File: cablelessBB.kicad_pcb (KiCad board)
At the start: 2 copper layers, 100 x 60 mm, 306 parts

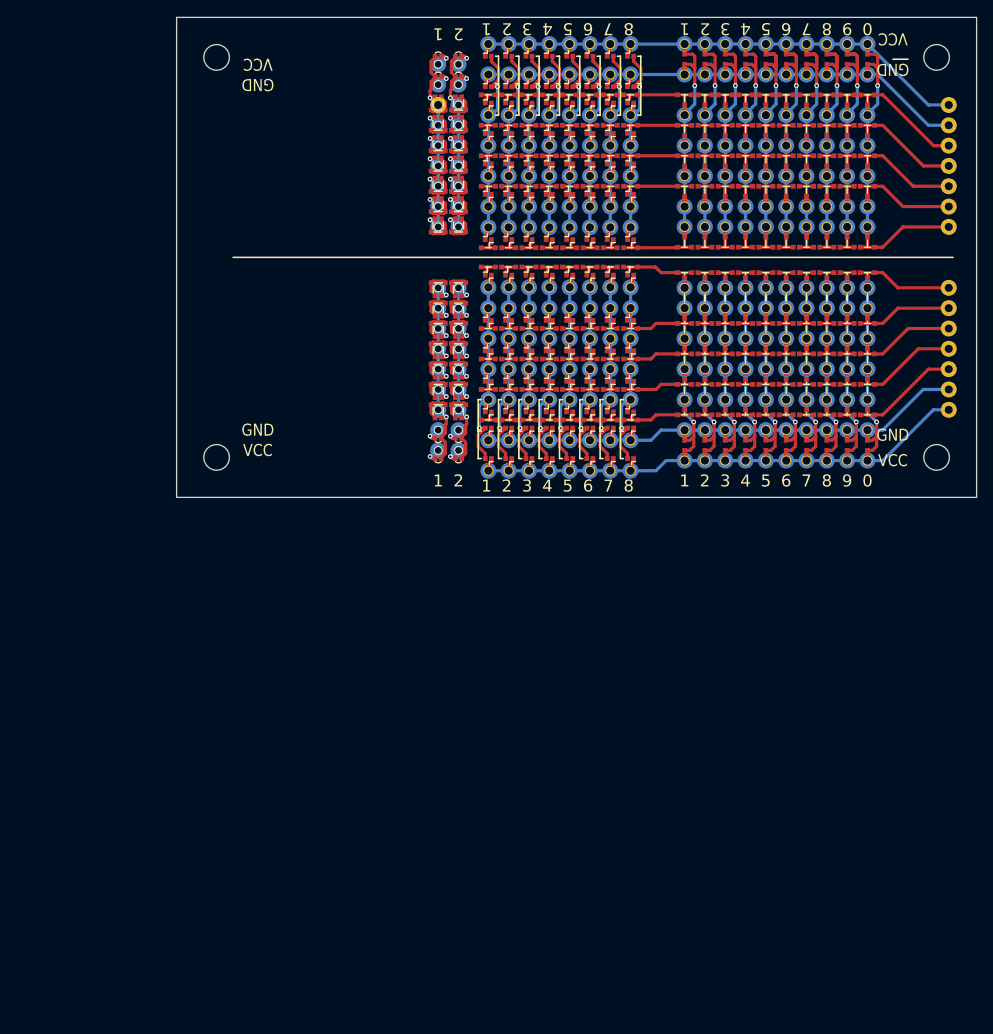
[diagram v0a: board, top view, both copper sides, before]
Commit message: 配線1
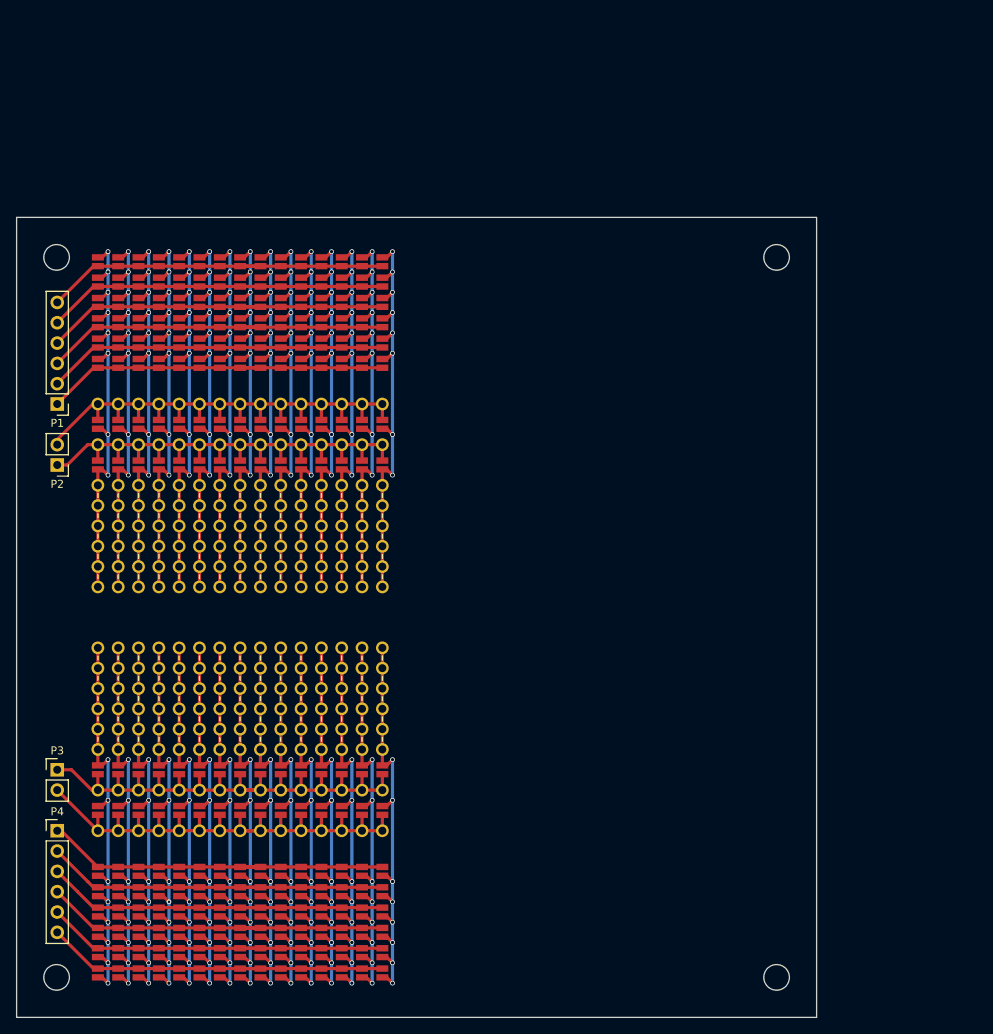
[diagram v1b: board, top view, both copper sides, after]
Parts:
- removed the REF** at (159.0, 72.8)
- removed the REF** at (161.5, 65.2)
- removed the REF** at (174.2, 32.1)
- removed the REF** at (174.2, 41.0)
- removed the REF** at (174.2, 48.6)
- removed the REF** at (174.2, 44.8)
- removed the REF** at (174.2, 51.3)
- removed the REF** at (174.2, 28.3)
- removed the REF** at (176.8, 28.3)
- removed the REF** at (176.8, 51.3)
- removed the REF** at (176.8, 44.8)
- removed the REF** at (176.8, 48.6)
- removed the REF** at (161.5, 61.4)
- removed the REF** at (176.8, 41.0)
- removed the REF** at (216.5, 58.8)
- removed the REF** at (216.5, 61.4)
- removed the REF** at (216.5, 66.4)
- removed the REF** at (216.5, 63.9)
- removed the REF** at (216.5, 74.0)
- removed the REF** at (216.5, 71.5)
- removed the REF** at (216.5, 69.0)
- removed the REF** at (216.5, 46.1)
- removed the REF** at (216.5, 48.6)
- removed the REF** at (161.5, 69.0)
- removed the REF** at (216.5, 51.2)
- removed the REF** at (216.5, 41.0)
- removed the REF** at (216.5, 43.6)
- removed the REF** at (216.5, 38.5)
- removed the REF** at (188.6, 51.2)
- removed the REF** at (188.6, 48.6)
- removed the REF** at (188.6, 44.8)
- removed the REF** at (188.6, 37.2)
- removed the REF** at (188.6, 41.0)
- removed the REF** at (188.6, 32.1)
- removed the REF** at (161.5, 77.9)
- removed the REF** at (201.3, 28.3)
- removed the REF** at (191.1, 41.0)
- removed the REF** at (191.1, 44.8)
- removed the REF** at (191.1, 48.6)
- removed the REF** at (191.1, 51.2)
- removed the REF** at (203.8, 28.3)
- removed the REF** at (191.1, 32.1)
- removed the REF** at (191.1, 37.2)
- removed the REF** at (196.2, 37.2)
- removed the REF** at (196.2, 32.1)
- removed the REF** at (161.5, 72.8)
- removed the REF** at (196.2, 51.2)
- removed the REF** at (196.2, 48.6)
- removed the REF** at (196.2, 44.8)
- removed the REF** at (196.2, 41.0)
- removed the REF** at (193.7, 32.1)
- removed the REF** at (193.7, 41.0)
- removed the REF** at (193.7, 37.2)
- removed the REF** at (193.7, 44.8)
- removed the REF** at (193.7, 48.6)
- removed the REF** at (193.7, 51.2)
- removed the REF** at (166.6, 72.8)
- removed the REF** at (203.8, 51.2)
- removed the REF** at (203.8, 48.6)
- removed the REF** at (203.8, 44.8)
- removed the REF** at (203.8, 37.2)
- removed the REF** at (203.8, 41.0)
- removed the REF** at (203.8, 32.1)
- removed the REF** at (206.4, 41.0)
- removed the REF** at (206.4, 44.8)
- removed the REF** at (206.4, 48.6)
- removed the REF** at (206.4, 51.2)
- removed the REF** at (166.6, 77.9)
- removed the REF** at (206.4, 28.3)
- removed the REF** at (206.4, 32.1)
- removed the REF** at (206.4, 37.2)
- removed the REF** at (201.3, 37.2)
- removed the REF** at (201.3, 32.1)
- removed the REF** at (201.3, 51.2)
- removed the REF** at (201.3, 48.6)
- removed the REF** at (201.3, 44.8)
- removed the REF** at (201.3, 41.0)
- removed the REF** at (198.7, 32.1)
- removed the REF** at (166.6, 69.0)
- removed the REF** at (198.7, 41.0)
- removed the REF** at (198.7, 37.2)
- removed the REF** at (198.7, 44.8)
- removed the REF** at (198.7, 48.6)
- removed the REF** at (198.7, 51.2)
- removed the REF** at (191.1, 28.3)
- removed the REF** at (193.7, 28.3)
- removed the REF** at (186.0, 37.2)
- removed the REF** at (186.0, 32.1)
- removed the REF** at (198.7, 28.3)
- removed the REF** at (166.6, 61.4)
- removed the REF** at (186.0, 51.2)
- removed the REF** at (186.0, 48.6)
- removed the REF** at (186.0, 44.8)
- removed the REF** at (186.0, 41.0)
- removed the REF** at (196.2, 28.3)
- removed the REF** at (183.5, 32.1)
- removed the REF** at (183.5, 41.0)
- removed the REF** at (183.5, 37.2)
- removed the REF** at (183.5, 44.8)
- removed the REF** at (183.5, 48.6)
- removed the REF** at (166.6, 65.2)
- removed the REF** at (183.5, 51.2)
- removed the REF** at (186.0, 28.3)
- removed the REF** at (188.6, 28.3)
- removed the REF** at (183.5, 28.3)
- removed the REF** at (188.6, 76.6)
- removed the REF** at (188.6, 80.4)
- removed the REF** at (191.1, 80.4)
- removed the REF** at (191.1, 76.6)
- removed the REF** at (196.2, 76.6)
- removed the REF** at (196.2, 80.4)
- removed the REF** at (159.0, 77.9)
- removed the REF** at (166.6, 58.7)
- removed the REF** at (193.7, 80.4)
- removed the REF** at (193.7, 76.6)
- removed the REF** at (203.8, 76.6)
- removed the REF** at (203.8, 80.4)
- removed the REF** at (206.4, 80.4)
- removed the REF** at (206.4, 76.6)
- removed the REF** at (201.3, 76.6)
- removed the REF** at (201.3, 80.4)
- removed the REF** at (198.7, 80.4)
- removed the REF** at (198.7, 76.6)
- removed the REF** at (166.6, 81.7)
- removed the REF** at (186.0, 76.6)
- removed the REF** at (186.0, 80.4)
- removed the REF** at (183.5, 80.4)
- removed the REF** at (183.5, 76.6)
- removed the REF** at (188.6, 58.8)
- removed the REF** at (188.6, 61.4)
- removed the REF** at (164.1, 81.7)
- removed the REF** at (188.6, 65.2)
- removed the REF** at (188.6, 72.8)
- removed the REF** at (188.6, 69.0)
- removed the REF** at (191.1, 69.0)
- removed the REF** at (191.1, 72.8)
- removed the REF** at (191.1, 65.2)
- removed the REF** at (191.1, 61.4)
- removed the REF** at (191.1, 58.8)
- removed the REF** at (196.2, 58.8)
- removed the REF** at (196.2, 61.4)
- removed the REF** at (164.1, 58.7)
- removed the REF** at (196.2, 65.2)
- removed the REF** at (196.2, 72.8)
- removed the REF** at (196.2, 69.0)
- removed the REF** at (193.7, 69.0)
- removed the REF** at (193.7, 72.8)
- removed the REF** at (193.7, 65.2)
- removed the REF** at (193.7, 61.4)
- removed the REF** at (193.7, 58.8)
- removed the REF** at (203.8, 58.8)
- removed the REF** at (203.8, 61.4)
- removed the REF** at (164.1, 65.2)
- removed the REF** at (203.8, 65.2)
- removed the REF** at (203.8, 72.8)
- removed the REF** at (203.8, 69.0)
- removed the REF** at (206.4, 69.0)
- removed the REF** at (206.4, 72.8)
- removed the REF** at (206.4, 65.2)
- removed the REF** at (206.4, 61.4)
- removed the REF** at (206.4, 58.8)
- removed the REF** at (201.3, 58.8)
- removed the REF** at (201.3, 61.4)
- removed the REF** at (164.1, 61.4)
- removed the REF** at (201.3, 65.2)
- removed the REF** at (201.3, 72.8)
- removed the REF** at (201.3, 69.0)
- removed the REF** at (198.7, 69.0)
- removed the REF** at (198.7, 72.8)
- removed the REF** at (198.7, 65.2)
- removed the REF** at (198.7, 61.4)
- removed the REF** at (198.7, 58.8)
- removed the REF** at (186.0, 58.8)
- removed the REF** at (186.0, 61.4)
- removed the REF** at (164.1, 69.0)
- removed the REF** at (186.0, 65.2)
- removed the REF** at (186.0, 72.8)
- removed the REF** at (186.0, 69.0)
- removed the REF** at (183.5, 69.0)
- removed the REF** at (183.5, 72.8)
- removed the REF** at (183.5, 65.2)
- removed the REF** at (183.5, 61.4)
- removed the REF** at (183.5, 58.8)
- removed the REF** at (216.5, 36.0)
- removed the REF** at (152.7, 46.1)
- removed the REF** at (164.1, 77.9)
- removed the REF** at (152.7, 48.6)
- removed the REF** at (152.7, 38.5)
- removed the REF** at (152.7, 36.0)
- removed the REF** at (152.7, 41.0)
- removed the REF** at (152.7, 43.6)
- removed the REF** at (152.7, 51.2)
- removed the REF** at (155.2, 51.2)
- removed the REF** at (155.2, 43.6)
- removed the REF** at (155.2, 41.0)
- removed the REF** at (155.2, 36.0)
- removed the REF** at (164.1, 72.8)
- removed the REF** at (155.2, 38.5)
- removed the REF** at (155.2, 48.6)
- removed the REF** at (155.2, 46.1)
- removed the REF** at (155.2, 63.9)
- removed the REF** at (155.2, 61.4)
- removed the REF** at (155.2, 71.5)
- removed the REF** at (155.2, 74.0)
- removed the REF** at (155.2, 69.0)
- removed the REF** at (155.2, 66.4)
- removed the REF** at (155.2, 58.8)
- removed the REF** at (174.2, 72.8)
- removed the REF** at (152.7, 58.8)
- removed the REF** at (152.7, 66.4)
- removed the REF** at (152.7, 69.0)
- removed the REF** at (152.7, 74.0)
- removed the REF** at (152.7, 71.5)
- removed the REF** at (152.7, 61.4)
- removed the REF** at (152.7, 63.9)
- removed the REF** at (152.7, 33.4)
- removed the REF** at (152.7, 30.9)
- removed the REF** at (155.2, 30.9)
- removed the REF** at (159.0, 69.0)
- removed the REF** at (174.2, 77.9)
- removed the REF** at (155.2, 33.4)
- removed the REF** at (155.2, 76.6)
- removed the REF** at (155.2, 79.1)
- removed the REF** at (152.7, 79.1)
- removed the REF** at (152.7, 76.6)
- removed the REF** at (176.8, 32.1)
- removed the REF** at (176.8, 37.2)
- removed the REF** at (174.2, 69.0)
- removed the REF** at (174.2, 61.4)
- removed the REF** at (174.2, 65.2)
- removed the REF** at (174.2, 58.7)
- removed the REF** at (174.2, 81.7)
- removed the REF** at (176.8, 81.7)
- removed the REF** at (176.8, 58.7)
- removed the REF** at (176.8, 65.2)
- removed the REF** at (176.8, 61.4)
- removed the REF** at (159.0, 61.4)
- removed the REF** at (176.8, 69.0)
- removed the REF** at (176.8, 77.9)
- removed the REF** at (176.8, 72.8)
- removed the REF** at (171.7, 72.8)
- removed the REF** at (171.7, 77.9)
- removed the REF** at (171.7, 69.0)
- removed the REF** at (171.7, 61.4)
- removed the REF** at (171.7, 65.2)
- removed the REF** at (171.7, 58.7)
- removed the REF** at (171.7, 81.7)
- removed the REF** at (159.0, 65.2)
- removed the REF** at (169.1, 81.7)
- removed the REF** at (169.1, 58.7)
- removed the REF** at (169.1, 65.2)
- removed the REF** at (169.1, 61.4)
- removed the REF** at (169.1, 69.0)
- removed the REF** at (169.1, 77.9)
- removed the REF** at (169.1, 72.8)
- removed the REF** at (166.6, 37.2)
- removed the REF** at (166.6, 32.1)
- removed the REF** at (166.6, 41.0)
- removed the REF** at (159.0, 58.7)
- removed the REF** at (166.6, 48.6)
- removed the REF** at (166.6, 44.8)
- removed the REF** at (166.6, 51.3)
- removed the REF** at (166.6, 28.3)
- removed the REF** at (164.1, 28.3)
- removed the REF** at (164.1, 51.3)
- removed the REF** at (164.1, 44.8)
- removed the REF** at (164.1, 48.6)
- removed the REF** at (164.1, 41.0)
- removed the REF** at (164.1, 32.1)
- removed the REF** at (159.0, 81.7)
- removed the REF** at (164.1, 37.2)
- removed the REF** at (159.0, 37.2)
- removed the REF** at (159.0, 32.1)
- removed the REF** at (159.0, 41.0)
- removed the REF** at (159.0, 48.6)
- removed the REF** at (159.0, 44.8)
- removed the REF** at (159.0, 51.3)
- removed the REF** at (159.0, 28.3)
- removed the REF** at (161.5, 28.3)
- removed the REF** at (161.5, 51.3)
- removed the REF** at (161.5, 81.7)
- removed the REF** at (161.5, 44.8)
- removed the REF** at (161.5, 48.6)
- removed the REF** at (161.5, 41.0)
- removed the REF** at (161.5, 32.1)
- removed the REF** at (161.5, 37.2)
- removed the REF** at (171.7, 37.2)
- removed the REF** at (171.7, 32.1)
- removed the REF** at (171.7, 41.0)
- removed the REF** at (171.7, 48.6)
- removed the REF** at (171.7, 44.8)
- removed the REF** at (161.5, 58.7)
- removed the REF** at (171.7, 51.3)
- removed the REF** at (171.7, 28.3)
- removed the REF** at (169.1, 28.3)
- removed the REF** at (169.1, 51.3)
- removed the REF** at (169.1, 44.8)
- removed the REF** at (169.1, 48.6)
- removed the REF** at (169.1, 41.0)
- removed the REF** at (169.1, 32.1)
- removed the REF** at (169.1, 37.2)
- removed the REF** at (174.2, 37.2)
- added JP1: Jumper_NO_Small, lib:jump, F.Cu at (110.2, 55.5)
- added JP10: Jumper_NO_Small, lib:jump, F.Cu at (110.2, 124.1)
- added JP100: Jumper_NO_Small, lib:jump, F.Cu at (125.4, 63.2)
- added JP101: Jumper_NO_Small, lib:jump, F.Cu at (125.4, 65.7)
- added JP102: Jumper_NO_Small, lib:jump, F.Cu at (125.4, 68.2)
- added JP103: Jumper_NO_Small, lib:jump, F.Cu at (125.4, 75.9)
- added JP104: Jumper_NO_Small, lib:jump, F.Cu at (125.4, 81.0)
- added JP105: Jumper_NO_Small, lib:jump, F.Cu at (125.4, 119.0)
- added JP106: Jumper_NO_Small, lib:jump, F.Cu at (125.4, 124.1)
- added JP107: Jumper_NO_Small, lib:jump, F.Cu at (125.4, 131.8)
- added JP108: Jumper_NO_Small, lib:jump, F.Cu at (125.4, 134.3)
- added JP109: Jumper_NO_Small, lib:jump, F.Cu at (125.4, 136.8)
- added JP11: Jumper_NO_Small, lib:jump, F.Cu at (110.2, 131.8)
- added JP110: Jumper_NO_Small, lib:jump, F.Cu at (125.4, 139.4)
- added JP111: Jumper_NO_Small, lib:jump, F.Cu at (125.4, 141.9)
- added JP112: Jumper_NO_Small, lib:jump, F.Cu at (125.4, 144.4)
- added JP113: Jumper_NO_Small, lib:jump, F.Cu at (127.9, 55.5)
- added JP114: Jumper_NO_Small, lib:jump, F.Cu at (127.9, 58.1)
- added JP115: Jumper_NO_Small, lib:jump, F.Cu at (127.9, 60.6)
- added JP116: Jumper_NO_Small, lib:jump, F.Cu at (127.9, 63.2)
- added JP117: Jumper_NO_Small, lib:jump, F.Cu at (127.9, 65.7)
- added JP118: Jumper_NO_Small, lib:jump, F.Cu at (127.9, 68.2)
- added JP119: Jumper_NO_Small, lib:jump, F.Cu at (127.9, 75.9)
- added JP12: Jumper_NO_Small, lib:jump, F.Cu at (110.2, 134.3)
- added JP120: Jumper_NO_Small, lib:jump, F.Cu at (127.9, 81.0)
- added JP121: Jumper_NO_Small, lib:jump, F.Cu at (127.9, 119.0)
- added JP122: Jumper_NO_Small, lib:jump, F.Cu at (127.9, 124.1)
- added JP123: Jumper_NO_Small, lib:jump, F.Cu at (127.9, 131.8)
- added JP124: Jumper_NO_Small, lib:jump, F.Cu at (127.9, 134.3)
- added JP125: Jumper_NO_Small, lib:jump, F.Cu at (127.9, 136.8)
- added JP126: Jumper_NO_Small, lib:jump, F.Cu at (127.9, 139.4)
- added JP127: Jumper_NO_Small, lib:jump, F.Cu at (127.9, 141.9)
- added JP128: Jumper_NO_Small, lib:jump, F.Cu at (127.9, 144.4)
- added JP129: Jumper_NO_Small, lib:jump, F.Cu at (130.5, 55.5)
- added JP13: Jumper_NO_Small, lib:jump, F.Cu at (110.2, 136.8)
- added JP130: Jumper_NO_Small, lib:jump, F.Cu at (130.5, 58.1)
- added JP131: Jumper_NO_Small, lib:jump, F.Cu at (130.5, 60.6)
- added JP132: Jumper_NO_Small, lib:jump, F.Cu at (130.5, 63.2)
- added JP133: Jumper_NO_Small, lib:jump, F.Cu at (130.5, 65.7)
- added JP134: Jumper_NO_Small, lib:jump, F.Cu at (130.5, 68.2)
- added JP135: Jumper_NO_Small, lib:jump, F.Cu at (130.5, 75.9)
- added JP136: Jumper_NO_Small, lib:jump, F.Cu at (130.5, 81.0)
- added JP137: Jumper_NO_Small, lib:jump, F.Cu at (130.5, 119.0)
- added JP138: Jumper_NO_Small, lib:jump, F.Cu at (130.5, 124.1)
- added JP139: Jumper_NO_Small, lib:jump, F.Cu at (130.5, 131.8)
- added JP14: Jumper_NO_Small, lib:jump, F.Cu at (110.2, 139.4)
- added JP140: Jumper_NO_Small, lib:jump, F.Cu at (130.5, 134.3)
- added JP141: Jumper_NO_Small, lib:jump, F.Cu at (130.5, 136.8)
- added JP142: Jumper_NO_Small, lib:jump, F.Cu at (130.5, 139.4)
- added JP143: Jumper_NO_Small, lib:jump, F.Cu at (130.5, 141.9)
- added JP144: Jumper_NO_Small, lib:jump, F.Cu at (130.5, 144.4)
- added JP145: Jumper_NO_Small, lib:jump, F.Cu at (133.0, 55.5)
- added JP146: Jumper_NO_Small, lib:jump, F.Cu at (133.0, 58.1)
- added JP147: Jumper_NO_Small, lib:jump, F.Cu at (133.0, 60.6)
- added JP148: Jumper_NO_Small, lib:jump, F.Cu at (133.0, 63.2)
- added JP149: Jumper_NO_Small, lib:jump, F.Cu at (133.0, 65.7)
- added JP15: Jumper_NO_Small, lib:jump, F.Cu at (110.2, 141.9)
- added JP150: Jumper_NO_Small, lib:jump, F.Cu at (133.0, 68.2)
- added JP151: Jumper_NO_Small, lib:jump, F.Cu at (133.0, 75.9)
- added JP152: Jumper_NO_Small, lib:jump, F.Cu at (133.0, 81.0)
- added JP153: Jumper_NO_Small, lib:jump, F.Cu at (133.0, 119.0)
- added JP154: Jumper_NO_Small, lib:jump, F.Cu at (133.0, 124.1)
- added JP155: Jumper_NO_Small, lib:jump, F.Cu at (133.0, 131.8)
- added JP156: Jumper_NO_Small, lib:jump, F.Cu at (133.0, 134.3)
- added JP157: Jumper_NO_Small, lib:jump, F.Cu at (133.0, 136.8)
- added JP158: Jumper_NO_Small, lib:jump, F.Cu at (133.0, 139.4)
- added JP159: Jumper_NO_Small, lib:jump, F.Cu at (133.0, 141.9)
- added JP16: Jumper_NO_Small, lib:jump, F.Cu at (110.2, 144.4)
- added JP160: Jumper_NO_Small, lib:jump, F.Cu at (133.0, 144.4)
- added JP161: Jumper_NO_Small, lib:jump, F.Cu at (135.6, 55.5)
- added JP162: Jumper_NO_Small, lib:jump, F.Cu at (135.6, 58.1)
- added JP163: Jumper_NO_Small, lib:jump, F.Cu at (135.6, 60.6)
- added JP164: Jumper_NO_Small, lib:jump, F.Cu at (135.6, 63.2)
- added JP165: Jumper_NO_Small, lib:jump, F.Cu at (135.6, 65.7)
- added JP166: Jumper_NO_Small, lib:jump, F.Cu at (135.6, 68.2)
- added JP167: Jumper_NO_Small, lib:jump, F.Cu at (135.6, 75.9)
- added JP168: Jumper_NO_Small, lib:jump, F.Cu at (135.6, 81.0)
- added JP169: Jumper_NO_Small, lib:jump, F.Cu at (135.6, 119.0)
- added JP17: Jumper_NO_Small, lib:jump, F.Cu at (112.7, 55.5)
- added JP170: Jumper_NO_Small, lib:jump, F.Cu at (135.6, 124.1)
- added JP171: Jumper_NO_Small, lib:jump, F.Cu at (135.6, 131.8)
- added JP172: Jumper_NO_Small, lib:jump, F.Cu at (135.6, 134.3)
- added JP173: Jumper_NO_Small, lib:jump, F.Cu at (135.6, 136.8)
- added JP174: Jumper_NO_Small, lib:jump, F.Cu at (135.6, 139.4)
- added JP175: Jumper_NO_Small, lib:jump, F.Cu at (135.6, 141.9)
- added JP176: Jumper_NO_Small, lib:jump, F.Cu at (135.6, 144.4)
- added JP177: Jumper_NO_Small, lib:jump, F.Cu at (138.1, 55.5)
- added JP178: Jumper_NO_Small, lib:jump, F.Cu at (138.1, 58.1)
- added JP179: Jumper_NO_Small, lib:jump, F.Cu at (138.1, 60.6)
- added JP18: Jumper_NO_Small, lib:jump, F.Cu at (112.7, 58.1)
- added JP180: Jumper_NO_Small, lib:jump, F.Cu at (138.1, 63.2)
- added JP181: Jumper_NO_Small, lib:jump, F.Cu at (138.1, 65.7)
- added JP182: Jumper_NO_Small, lib:jump, F.Cu at (138.1, 68.2)
- added JP183: Jumper_NO_Small, lib:jump, F.Cu at (138.1, 75.9)
- added JP184: Jumper_NO_Small, lib:jump, F.Cu at (138.1, 81.0)
- added JP185: Jumper_NO_Small, lib:jump, F.Cu at (138.1, 119.0)
- added JP186: Jumper_NO_Small, lib:jump, F.Cu at (138.1, 124.1)
- added JP187: Jumper_NO_Small, lib:jump, F.Cu at (138.1, 131.8)
- added JP188: Jumper_NO_Small, lib:jump, F.Cu at (138.1, 134.3)
- added JP189: Jumper_NO_Small, lib:jump, F.Cu at (138.1, 136.8)
- added JP19: Jumper_NO_Small, lib:jump, F.Cu at (112.7, 60.6)
- added JP190: Jumper_NO_Small, lib:jump, F.Cu at (138.1, 139.4)
- added JP191: Jumper_NO_Small, lib:jump, F.Cu at (138.1, 141.9)
- added JP192: Jumper_NO_Small, lib:jump, F.Cu at (138.1, 144.4)
- added JP193: Jumper_NO_Small, lib:jump, F.Cu at (140.6, 55.5)
- added JP194: Jumper_NO_Small, lib:jump, F.Cu at (140.6, 58.1)
- added JP195: Jumper_NO_Small, lib:jump, F.Cu at (140.6, 60.6)
- added JP196: Jumper_NO_Small, lib:jump, F.Cu at (140.6, 63.2)
- added JP197: Jumper_NO_Small, lib:jump, F.Cu at (140.6, 65.7)
- added JP198: Jumper_NO_Small, lib:jump, F.Cu at (140.6, 68.2)
- added JP199: Jumper_NO_Small, lib:jump, F.Cu at (140.6, 75.9)
- added JP2: Jumper_NO_Small, lib:jump, F.Cu at (110.2, 58.1)
- added JP20: Jumper_NO_Small, lib:jump, F.Cu at (112.7, 63.2)
- added JP200: Jumper_NO_Small, lib:jump, F.Cu at (140.6, 81.0)
- added JP201: Jumper_NO_Small, lib:jump, F.Cu at (140.6, 119.0)
- added JP202: Jumper_NO_Small, lib:jump, F.Cu at (140.6, 124.1)
- added JP203: Jumper_NO_Small, lib:jump, F.Cu at (140.6, 131.8)
- added JP204: Jumper_NO_Small, lib:jump, F.Cu at (140.6, 134.3)
- added JP205: Jumper_NO_Small, lib:jump, F.Cu at (140.6, 136.8)
- added JP206: Jumper_NO_Small, lib:jump, F.Cu at (140.6, 139.4)
- added JP207: Jumper_NO_Small, lib:jump, F.Cu at (140.6, 141.9)
- added JP208: Jumper_NO_Small, lib:jump, F.Cu at (140.6, 144.4)
- added JP209: Jumper_NO_Small, lib:jump, F.Cu at (143.2, 55.5)
- added JP21: Jumper_NO_Small, lib:jump, F.Cu at (112.7, 65.7)
- added JP210: Jumper_NO_Small, lib:jump, F.Cu at (143.2, 58.1)
- added JP211: Jumper_NO_Small, lib:jump, F.Cu at (143.2, 60.6)
- added JP212: Jumper_NO_Small, lib:jump, F.Cu at (143.2, 63.2)
- added JP213: Jumper_NO_Small, lib:jump, F.Cu at (143.2, 65.7)
- added JP214: Jumper_NO_Small, lib:jump, F.Cu at (143.2, 68.2)
- added JP215: Jumper_NO_Small, lib:jump, F.Cu at (143.2, 75.9)
- added JP216: Jumper_NO_Small, lib:jump, F.Cu at (143.2, 81.0)
- added JP217: Jumper_NO_Small, lib:jump, F.Cu at (143.2, 119.0)
- added JP218: Jumper_NO_Small, lib:jump, F.Cu at (143.2, 124.1)
- added JP219: Jumper_NO_Small, lib:jump, F.Cu at (143.2, 131.8)
- added JP22: Jumper_NO_Small, lib:jump, F.Cu at (112.7, 68.2)
- added JP220: Jumper_NO_Small, lib:jump, F.Cu at (143.2, 134.3)
- added JP221: Jumper_NO_Small, lib:jump, F.Cu at (143.2, 136.8)
- added JP222: Jumper_NO_Small, lib:jump, F.Cu at (143.2, 139.4)
- added JP223: Jumper_NO_Small, lib:jump, F.Cu at (143.2, 141.9)
- added JP224: Jumper_NO_Small, lib:jump, F.Cu at (143.2, 144.4)
- added JP225: Jumper_NO_Small, lib:jump, F.Cu at (145.7, 55.5)
- added JP226: Jumper_NO_Small, lib:jump, F.Cu at (145.7, 58.1)
- added JP227: Jumper_NO_Small, lib:jump, F.Cu at (145.7, 60.6)
- added JP228: Jumper_NO_Small, lib:jump, F.Cu at (145.7, 63.2)
- added JP229: Jumper_NO_Small, lib:jump, F.Cu at (145.7, 65.7)
- added JP23: Jumper_NO_Small, lib:jump, F.Cu at (112.7, 75.9)
- added JP230: Jumper_NO_Small, lib:jump, F.Cu at (145.7, 68.2)
- added JP231: Jumper_NO_Small, lib:jump, F.Cu at (145.7, 75.9)
- added JP232: Jumper_NO_Small, lib:jump, F.Cu at (145.7, 81.0)
- added JP233: Jumper_NO_Small, lib:jump, F.Cu at (145.7, 119.0)
- added JP234: Jumper_NO_Small, lib:jump, F.Cu at (145.7, 124.1)
- added JP235: Jumper_NO_Small, lib:jump, F.Cu at (145.7, 131.8)
- added JP236: Jumper_NO_Small, lib:jump, F.Cu at (145.7, 134.3)
- added JP237: Jumper_NO_Small, lib:jump, F.Cu at (145.7, 136.8)
- added JP238: Jumper_NO_Small, lib:jump, F.Cu at (145.7, 139.4)
- added JP239: Jumper_NO_Small, lib:jump, F.Cu at (145.7, 141.9)
- added JP24: Jumper_NO_Small, lib:jump, F.Cu at (112.7, 81.0)
- added JP240: Jumper_NO_Small, lib:jump, F.Cu at (145.7, 144.4)
- added JP25: Jumper_NO_Small, lib:jump, F.Cu at (112.7, 119.0)
- added JP26: Jumper_NO_Small, lib:jump, F.Cu at (112.7, 124.1)
- added JP27: Jumper_NO_Small, lib:jump, F.Cu at (112.7, 131.8)
- added JP28: Jumper_NO_Small, lib:jump, F.Cu at (112.7, 134.3)
- added JP29: Jumper_NO_Small, lib:jump, F.Cu at (112.7, 136.8)
- added JP3: Jumper_NO_Small, lib:jump, F.Cu at (110.2, 60.6)
- added JP30: Jumper_NO_Small, lib:jump, F.Cu at (112.7, 139.4)
- added JP31: Jumper_NO_Small, lib:jump, F.Cu at (112.7, 141.9)
- added JP32: Jumper_NO_Small, lib:jump, F.Cu at (112.7, 144.4)
- added JP33: Jumper_NO_Small, lib:jump, F.Cu at (115.2, 55.5)
- added JP34: Jumper_NO_Small, lib:jump, F.Cu at (115.2, 58.1)
- added JP35: Jumper_NO_Small, lib:jump, F.Cu at (115.2, 60.6)
- added JP36: Jumper_NO_Small, lib:jump, F.Cu at (115.2, 63.2)
- added JP37: Jumper_NO_Small, lib:jump, F.Cu at (115.2, 65.7)
- added JP38: Jumper_NO_Small, lib:jump, F.Cu at (115.2, 68.2)
- added JP39: Jumper_NO_Small, lib:jump, F.Cu at (115.2, 75.9)
- added JP4: Jumper_NO_Small, lib:jump, F.Cu at (110.2, 63.2)
- added JP40: Jumper_NO_Small, lib:jump, F.Cu at (115.2, 81.0)
- added JP41: Jumper_NO_Small, lib:jump, F.Cu at (115.2, 119.0)
- added JP42: Jumper_NO_Small, lib:jump, F.Cu at (115.2, 124.1)
- added JP43: Jumper_NO_Small, lib:jump, F.Cu at (115.2, 131.8)
- added JP44: Jumper_NO_Small, lib:jump, F.Cu at (115.2, 134.3)
- added JP45: Jumper_NO_Small, lib:jump, F.Cu at (115.2, 136.8)
- added JP46: Jumper_NO_Small, lib:jump, F.Cu at (115.2, 139.4)
- added JP47: Jumper_NO_Small, lib:jump, F.Cu at (115.2, 141.9)
- added JP48: Jumper_NO_Small, lib:jump, F.Cu at (115.2, 144.4)
- added JP49: Jumper_NO_Small, lib:jump, F.Cu at (117.8, 55.5)
- added JP5: Jumper_NO_Small, lib:jump, F.Cu at (110.2, 65.7)
- added JP50: Jumper_NO_Small, lib:jump, F.Cu at (117.8, 58.1)
- added JP51: Jumper_NO_Small, lib:jump, F.Cu at (117.8, 60.6)
- added JP52: Jumper_NO_Small, lib:jump, F.Cu at (117.8, 63.2)
- added JP53: Jumper_NO_Small, lib:jump, F.Cu at (117.8, 65.7)
- added JP54: Jumper_NO_Small, lib:jump, F.Cu at (117.8, 68.2)
- added JP55: Jumper_NO_Small, lib:jump, F.Cu at (117.8, 75.9)
- added JP56: Jumper_NO_Small, lib:jump, F.Cu at (117.8, 81.0)
- added JP57: Jumper_NO_Small, lib:jump, F.Cu at (117.8, 119.0)
- added JP58: Jumper_NO_Small, lib:jump, F.Cu at (117.8, 124.1)
- added JP59: Jumper_NO_Small, lib:jump, F.Cu at (117.8, 131.8)
- added JP6: Jumper_NO_Small, lib:jump, F.Cu at (110.2, 68.2)
- added JP60: Jumper_NO_Small, lib:jump, F.Cu at (117.8, 134.3)
- added JP61: Jumper_NO_Small, lib:jump, F.Cu at (117.8, 136.8)
- added JP62: Jumper_NO_Small, lib:jump, F.Cu at (117.8, 139.4)
- added JP63: Jumper_NO_Small, lib:jump, F.Cu at (117.8, 141.9)
- added JP64: Jumper_NO_Small, lib:jump, F.Cu at (117.8, 144.4)
- added JP65: Jumper_NO_Small, lib:jump, F.Cu at (120.3, 55.5)
- added JP66: Jumper_NO_Small, lib:jump, F.Cu at (120.3, 58.1)
- added JP67: Jumper_NO_Small, lib:jump, F.Cu at (120.3, 60.6)
- added JP68: Jumper_NO_Small, lib:jump, F.Cu at (120.3, 63.2)
- added JP69: Jumper_NO_Small, lib:jump, F.Cu at (120.3, 65.7)
- added JP7: Jumper_NO_Small, lib:jump, F.Cu at (110.2, 75.9)
- added JP70: Jumper_NO_Small, lib:jump, F.Cu at (120.3, 68.2)
- added JP71: Jumper_NO_Small, lib:jump, F.Cu at (120.3, 75.9)
- added JP72: Jumper_NO_Small, lib:jump, F.Cu at (120.3, 81.0)
- added JP73: Jumper_NO_Small, lib:jump, F.Cu at (120.3, 119.0)
- added JP74: Jumper_NO_Small, lib:jump, F.Cu at (120.3, 124.1)
- added JP75: Jumper_NO_Small, lib:jump, F.Cu at (120.3, 131.8)
- added JP76: Jumper_NO_Small, lib:jump, F.Cu at (120.3, 134.3)
- added JP77: Jumper_NO_Small, lib:jump, F.Cu at (120.3, 136.8)
- added JP78: Jumper_NO_Small, lib:jump, F.Cu at (120.3, 139.4)
- added JP79: Jumper_NO_Small, lib:jump, F.Cu at (120.3, 141.9)
- added JP8: Jumper_NO_Small, lib:jump, F.Cu at (110.2, 81.0)
- added JP80: Jumper_NO_Small, lib:jump, F.Cu at (120.3, 144.4)
- added JP81: Jumper_NO_Small, lib:jump, F.Cu at (122.9, 55.5)
- added JP82: Jumper_NO_Small, lib:jump, F.Cu at (122.9, 58.1)
- added JP83: Jumper_NO_Small, lib:jump, F.Cu at (122.9, 60.6)
- added JP84: Jumper_NO_Small, lib:jump, F.Cu at (122.9, 63.2)
- added JP85: Jumper_NO_Small, lib:jump, F.Cu at (122.9, 65.7)
- added JP86: Jumper_NO_Small, lib:jump, F.Cu at (122.9, 68.2)
- added JP87: Jumper_NO_Small, lib:jump, F.Cu at (122.9, 75.9)
- added JP88: Jumper_NO_Small, lib:jump, F.Cu at (122.9, 81.0)
- added JP89: Jumper_NO_Small, lib:jump, F.Cu at (122.9, 119.0)
- added JP9: Jumper_NO_Small, lib:jump, F.Cu at (110.2, 119.0)
- added JP90: Jumper_NO_Small, lib:jump, F.Cu at (122.9, 124.1)
- added JP91: Jumper_NO_Small, lib:jump, F.Cu at (122.9, 131.8)
- added JP92: Jumper_NO_Small, lib:jump, F.Cu at (122.9, 134.3)
- added JP93: Jumper_NO_Small, lib:jump, F.Cu at (122.9, 136.8)
- added JP94: Jumper_NO_Small, lib:jump, F.Cu at (122.9, 139.4)
- added JP95: Jumper_NO_Small, lib:jump, F.Cu at (122.9, 141.9)
- added JP96: Jumper_NO_Small, lib:jump, F.Cu at (122.9, 144.4)
- added JP97: Jumper_NO_Small, lib:jump, F.Cu at (125.4, 55.5)
- added JP98: Jumper_NO_Small, lib:jump, F.Cu at (125.4, 58.1)
- added JP99: Jumper_NO_Small, lib:jump, F.Cu at (125.4, 60.6)
- added P1: CONN_01X06, Pin_Headers:Pin_Header_Straight_1x06_Pitch2.54mm, F.Cu at (105.1, 73.3)
- added P10: CONN_01X06, lib:6p, F.Cu at (112.7, 116.5)
- added P11: CONN_01X02, lib:2P, F.Cu at (112.7, 73.3)
- added P12: CONN_01X02, lib:2P, F.Cu at (112.7, 126.7)
- added P13: CONN_01X06, lib:6p, F.Cu at (115.2, 96.2)
- added P14: CONN_01X06, lib:6p, F.Cu at (115.2, 116.5)
- added P15: CONN_01X02, lib:2P, F.Cu at (115.2, 73.3)
- added P16: CONN_01X02, lib:2P, F.Cu at (115.2, 126.7)
- added P17: CONN_01X06, lib:6p, F.Cu at (117.8, 96.2)
- added P18: CONN_01X06, lib:6p, F.Cu at (117.8, 116.5)
- added P19: CONN_01X02, lib:2P, F.Cu at (117.8, 73.3)
- added P2: CONN_01X02, Pin_Headers:Pin_Header_Straight_1x02_Pitch2.54mm, F.Cu at (105.1, 81.0)
- added P20: CONN_01X02, lib:2P, F.Cu at (117.8, 126.7)
- added P21: CONN_01X06, lib:6p, F.Cu at (120.3, 96.2)
- added P22: CONN_01X06, lib:6p, F.Cu at (120.3, 116.5)
- added P23: CONN_01X02, lib:2P, F.Cu at (120.3, 73.3)
- added P24: CONN_01X02, lib:2P, F.Cu at (120.3, 126.7)
- added P25: CONN_01X06, lib:6p, F.Cu at (122.9, 96.2)
- added P26: CONN_01X06, lib:6p, F.Cu at (122.9, 116.5)
- added P27: CONN_01X02, lib:2P, F.Cu at (122.9, 73.3)
- added P28: CONN_01X02, lib:2P, F.Cu at (122.9, 126.7)
- added P29: CONN_01X06, lib:6p, F.Cu at (125.4, 96.2)
- added P3: CONN_01X02, Pin_Headers:Pin_Header_Straight_1x02_Pitch2.54mm, F.Cu at (105.1, 119.0)
- added P30: CONN_01X06, lib:6p, F.Cu at (125.4, 116.5)
- added P31: CONN_01X02, lib:2P, F.Cu at (125.4, 73.3)
- added P32: CONN_01X02, lib:2P, F.Cu at (125.4, 126.7)
- added P33: CONN_01X06, lib:6p, F.Cu at (127.9, 96.2)
- added P34: CONN_01X06, lib:6p, F.Cu at (127.9, 116.5)
- added P35: CONN_01X02, lib:2P, F.Cu at (127.9, 73.3)
- added P36: CONN_01X02, lib:2P, F.Cu at (127.9, 126.7)
- added P37: CONN_01X06, lib:6p, F.Cu at (130.5, 96.2)
- added P38: CONN_01X06, lib:6p, F.Cu at (130.5, 116.5)
- added P39: CONN_01X02, lib:2P, F.Cu at (130.5, 73.3)
- added P4: CONN_01X06, Pin_Headers:Pin_Header_Straight_1x06_Pitch2.54mm, F.Cu at (105.1, 126.7)
- added P40: CONN_01X02, lib:2P, F.Cu at (130.5, 126.7)
- added P41: CONN_01X06, lib:6p, F.Cu at (133.0, 96.2)
- added P42: CONN_01X06, lib:6p, F.Cu at (133.0, 116.5)
- added P43: CONN_01X02, lib:2P, F.Cu at (133.0, 73.3)
- added P44: CONN_01X02, lib:2P, F.Cu at (133.0, 126.7)
- added P45: CONN_01X06, lib:6p, F.Cu at (135.6, 96.2)
- added P46: CONN_01X06, lib:6p, F.Cu at (135.6, 116.5)
- added P47: CONN_01X02, lib:2P, F.Cu at (135.6, 73.3)
- added P48: CONN_01X02, lib:2P, F.Cu at (135.6, 126.7)
- added P49: CONN_01X06, lib:6p, F.Cu at (138.1, 96.2)
- added P5: CONN_01X06, lib:6p, F.Cu at (110.2, 96.2)
- added P50: CONN_01X06, lib:6p, F.Cu at (138.1, 116.5)
- added P51: CONN_01X02, lib:2P, F.Cu at (138.1, 73.3)
- added P52: CONN_01X02, lib:2P, F.Cu at (138.1, 126.7)
- added P53: CONN_01X06, lib:6p, F.Cu at (140.6, 96.2)
- added P54: CONN_01X06, lib:6p, F.Cu at (140.6, 116.5)
- added P55: CONN_01X02, lib:2P, F.Cu at (140.6, 73.3)
- added P56: CONN_01X02, lib:2P, F.Cu at (140.6, 126.7)
- added P57: CONN_01X06, lib:6p, F.Cu at (143.2, 96.2)
- added P58: CONN_01X06, lib:6p, F.Cu at (143.2, 116.5)
- added P59: CONN_01X02, lib:2P, F.Cu at (143.2, 73.3)
- added P6: CONN_01X06, lib:6p, F.Cu at (110.2, 116.5)
- added P60: CONN_01X02, lib:2P, F.Cu at (143.2, 126.7)
- added P61: CONN_01X06, lib:6p, F.Cu at (145.7, 96.2)
- added P62: CONN_01X06, lib:6p, F.Cu at (145.7, 116.5)
- added P63: CONN_01X02, lib:2P, F.Cu at (145.7, 73.3)
- added P64: CONN_01X02, lib:2P, F.Cu at (145.7, 126.7)
- added P7: CONN_01X02, lib:2P, F.Cu at (110.2, 73.3)
- added P8: CONN_01X02, lib:2P, F.Cu at (110.2, 126.7)
- added P9: CONN_01X06, lib:6p, F.Cu at (112.7, 96.2)
- moved REF** 68.0 mm to (195.0, 145.0)
- moved REF** 68.0 mm to (105.0, 145.0)
- moved REF** 32.0 mm to (105.0, 55.0)
- moved REF** 32.0 mm to (195.0, 55.0)
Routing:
- net GND: track 2229.4 -> 156.3 mm, vias 72 -> 0
- net VCC: track 0.00 -> 148.1 mm
- net Net-(JP233-Pad2): track 0.00 -> 55.2 mm, vias 0 -> 8
- net Net-(JP185-Pad2): track 0.00 -> 55.2 mm, vias 0 -> 8
- net Net-(JP177-Pad2): track 0.00 -> 55.2 mm, vias 0 -> 8
- net Net-(JP137-Pad2): track 0.00 -> 55.2 mm, vias 0 -> 8
- net Net-(JP129-Pad2): track 0.00 -> 55.2 mm, vias 0 -> 8
- net Net-(JP225-Pad2): track 0.00 -> 55.2 mm, vias 0 -> 8
- net Net-(JP73-Pad2): track 0.00 -> 55.2 mm, vias 0 -> 8
- net Net-(JP65-Pad2): track 0.00 -> 55.2 mm, vias 0 -> 8
- net Net-(JP41-Pad2): track 0.00 -> 55.2 mm, vias 0 -> 8
- net Net-(JP33-Pad2): track 0.00 -> 55.2 mm, vias 0 -> 8
- net Net-(JP201-Pad2): track 0.00 -> 55.2 mm, vias 0 -> 8
- net Net-(JP193-Pad2): track 0.00 -> 55.2 mm, vias 0 -> 8
- net Net-(JP169-Pad2): track 0.00 -> 55.2 mm, vias 0 -> 8
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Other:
- board size 100 x 60 mm -> 100 x 100 mm
- net class AC100V removed
- net class Default: clearance 0.2 -> 0.19; via_drill 0.4 -> 0.3
- net class VCC removed
- net class vm5V removed
- rule trace_clearance: 0.2 -> 0.19
- board text removed: "0"
- board text removed: "1"
- board text removed: "2"
- board text removed: "3"
- board text removed: "4"
- board text removed: "5"
- board text removed: "6"
- board text removed: "7"
- board text removed: "8"
- board text removed: "9"
- board text removed: "GND"
- board text removed: "VCC"
